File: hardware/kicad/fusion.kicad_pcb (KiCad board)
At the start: 2 copper layers, 133.6 x 59.7 mm, 32 parts, among them J1 BATTERY, J2 LSM6DSOX, J3 PICKIT, J4 HC-05, J5 FLEX, J7 FTDI, SW1 BUTTON, SW2 POWER, SW3 UART, U1 MCP1603, U2 PIC16F690

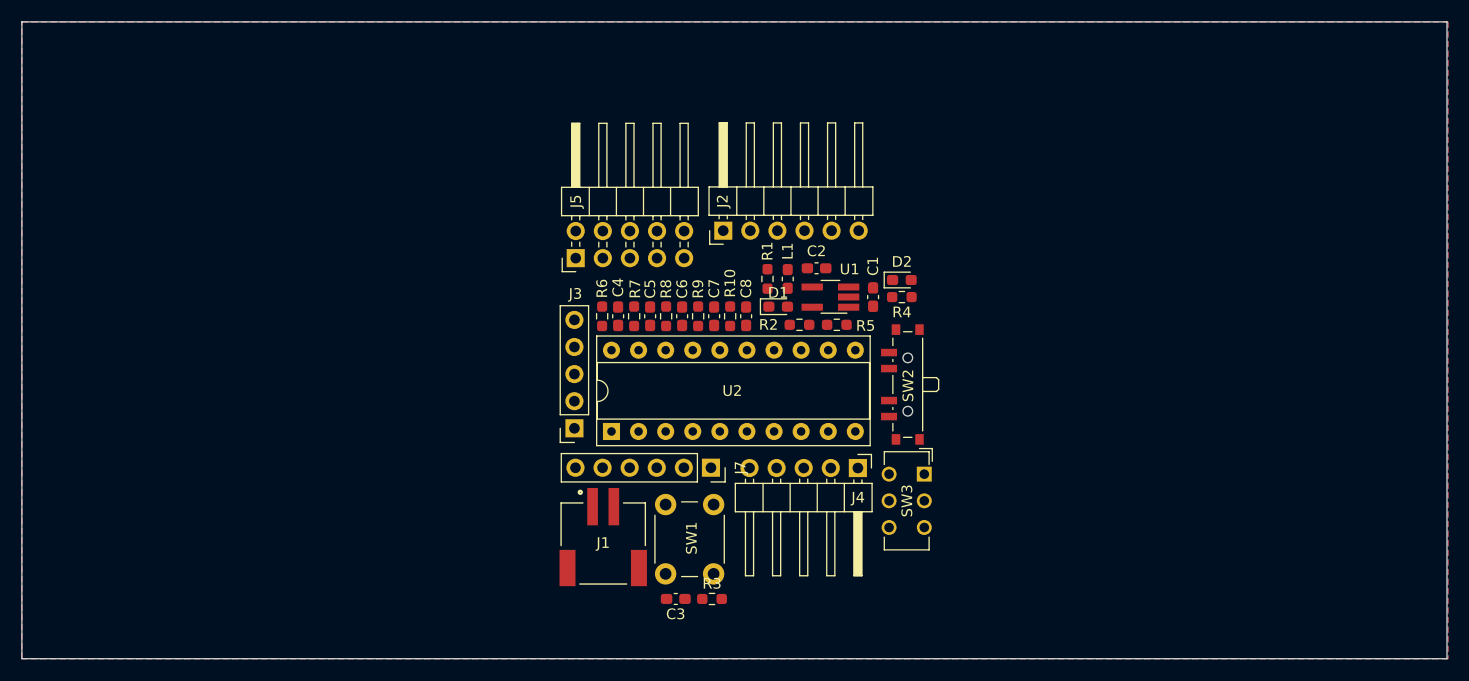
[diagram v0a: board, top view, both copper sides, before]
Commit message: Route board
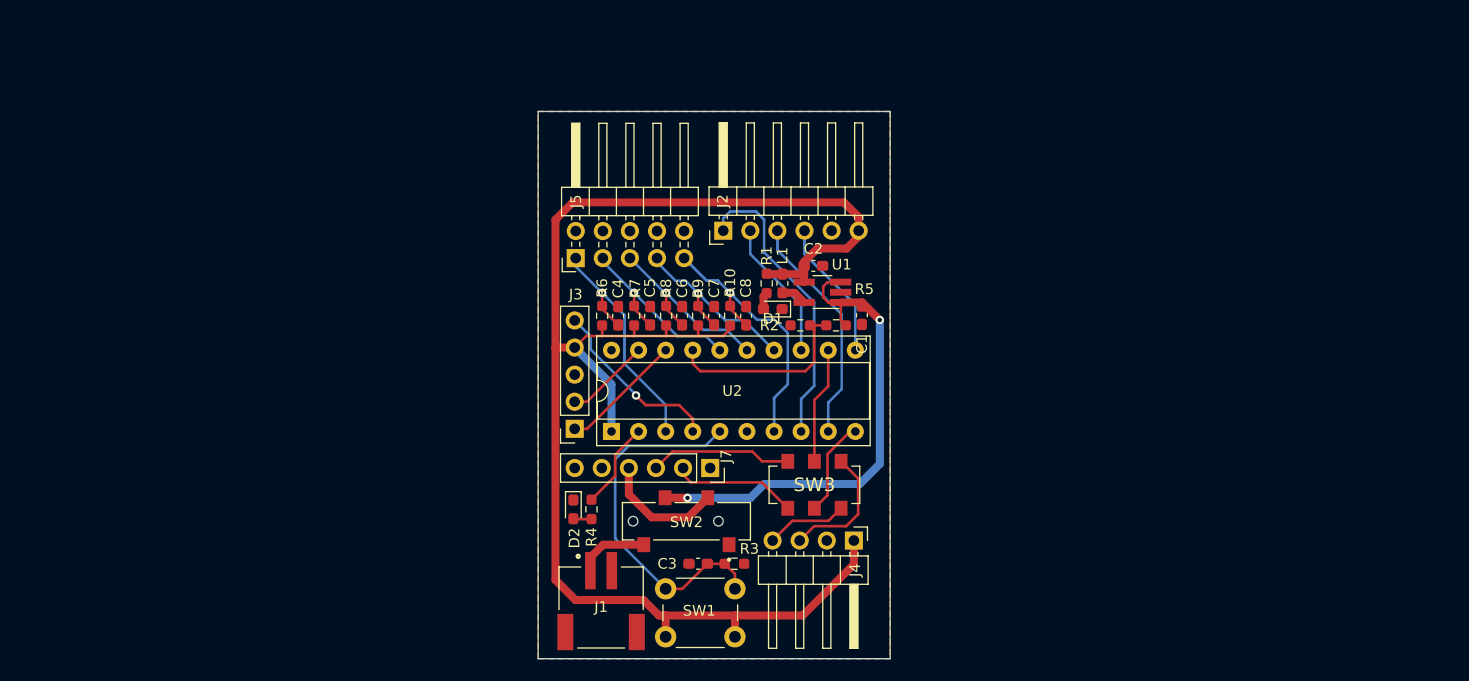
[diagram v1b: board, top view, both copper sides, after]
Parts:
- J4: footprint Connector_PinHeader_2.54mm:PinHeader_1x05_P2.54mm_Horizontal -> Connector_PinHeader_2.54mm:PinHeader_1x04_P2.54mm_Horizontal
- SW2: footprint Button_Switch_SMD:SW_SP3T_PCM13 -> Fusion:SP3T
- SW3: footprint Button_Switch_THT:SW_CuK_JS202011CQN_DPDT_Straight -> Fusion:SPDT
- moved D2 37.6 mm to (140.3, 105.3), turned to -90 degrees
- moved R4 35.3 mm to (142.0, 105.3), turned to 90 degrees
- moved SW2 24.1 mm to (150.9, 106.4), turned to 180 degrees
- moved SW3 10.3 mm to (162.9, 103.0), turned to 180 degrees
- moved SW1 9.09 mm to (148.9, 112.8), turned to 0 degrees
- moved J4 6.81 mm to (166.6, 108.2)
- moved J1 6.00 mm to (142.9, 111.0)
- moved C3 3.91 mm to (152.0, 110.4)
- moved R3 3.91 mm to (155.4, 110.4)
- moved C1 2.00 mm to (167.3, 87.1)
- moved U1 0.87 mm to (163.7, 85.0)
- moved L1 0.66 mm to (159.9, 84.1)
- moved D1 0.55 mm to (159.0, 86.5), turned to 180 degrees
- moved R1 0.43 mm to (158.4, 84.1)
- moved C2 0.37 mm to (162.8, 82.5)
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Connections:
- J4 pad 1: BT_KEY -> +3V3
- J4 pad 2: +3V3 -> GNDREF
- J4 pad 3: GNDREF -> BT_TX
- J4 pad 4: BT_TX -> BT_RX
- U2 pad 2: BT_KEY -> LED
- U2 pad 6: LED -> unconnected-(U2-Pad6)
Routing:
- net +3V3: track 0.00 -> 145.2 mm
- net Net-(C1-Pad1): track 0.00 -> 46.3 mm, vias 0 -> 2
- net BUTTON: track 0.00 -> 34.3 mm
- net CS: track 0.00 -> 27.9 mm
- net PINKY: track 0.00 -> 26.0 mm, vias 0 -> 1
- net THUMB: track 0.00 -> 23.4 mm, vias 0 -> 1
- net MOSI: track 0.00 -> 21.8 mm
- net VBAT_ADC: track 0.00 -> 18.8 mm
- net INDEX: track 0.00 -> 18.4 mm, vias 0 -> 1
- net RING: track 0.00 -> 18.4 mm, vias 0 -> 1
- net MIDDLE: track 0.00 -> 18.2 mm, vias 0 -> 1
- net MCLR: track 0.00 -> 16.8 mm, vias 0 -> 1
- net FTDI_TX: track 0.00 -> 13.4 mm
- net SCK: track 0.00 -> 13.2 mm
- net MISO: track 0.00 -> 13.2 mm
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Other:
- board size 133.6 x 59.7 mm -> 33 x 51.3 mm
